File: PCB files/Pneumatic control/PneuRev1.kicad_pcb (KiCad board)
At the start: 2 copper layers, 154.1 x 77.3 mm, 76 parts, among them J1 SIG_IN, J2 BATT_IN, J3 PNEU, U1 OPA551, U10 OPA551, U11 OPA551, U12 OPA551, U13 OPA551, U2 OPA551, U3 OPA551, U4 OPA551, U5 OPA551, U6 OPA551, U7 OPA551, U8 OPA551, U9 OPA551

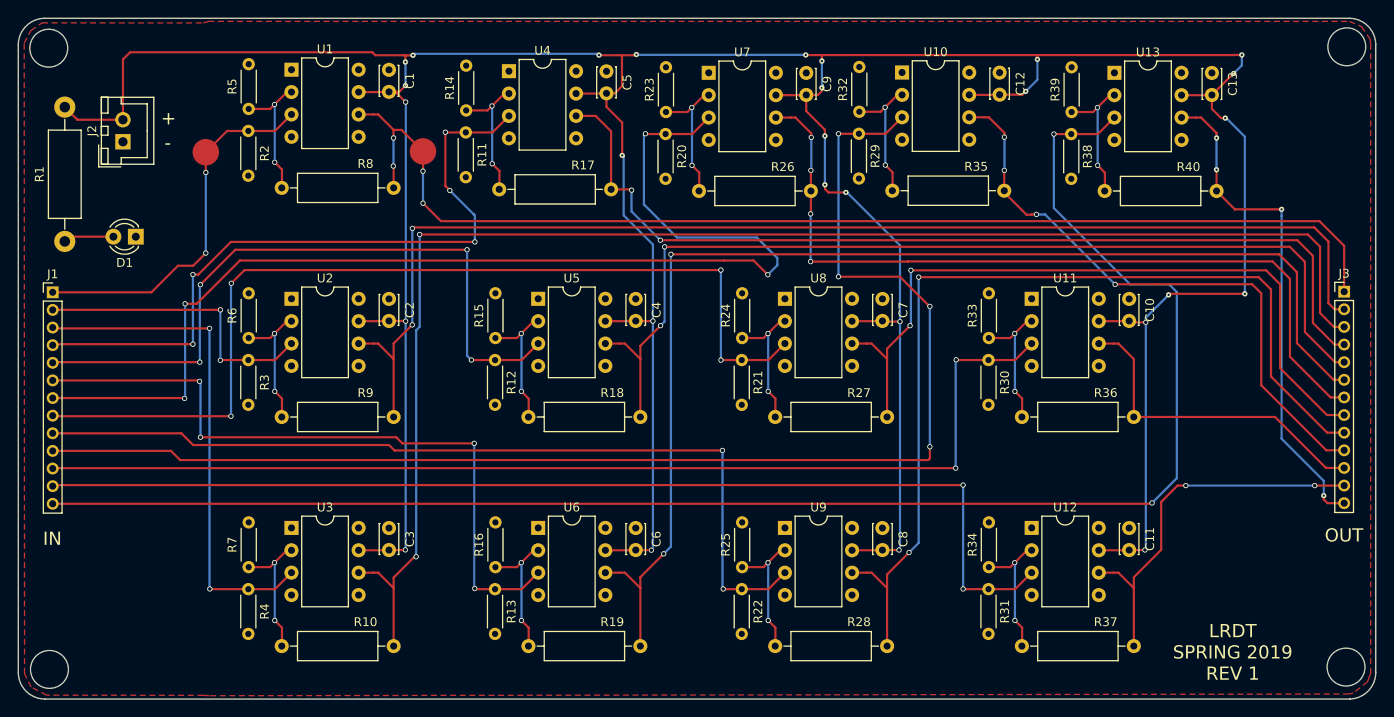
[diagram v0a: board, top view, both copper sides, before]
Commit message: 12/10/2019
-Selected battery molex connector footprint
-Read netlist
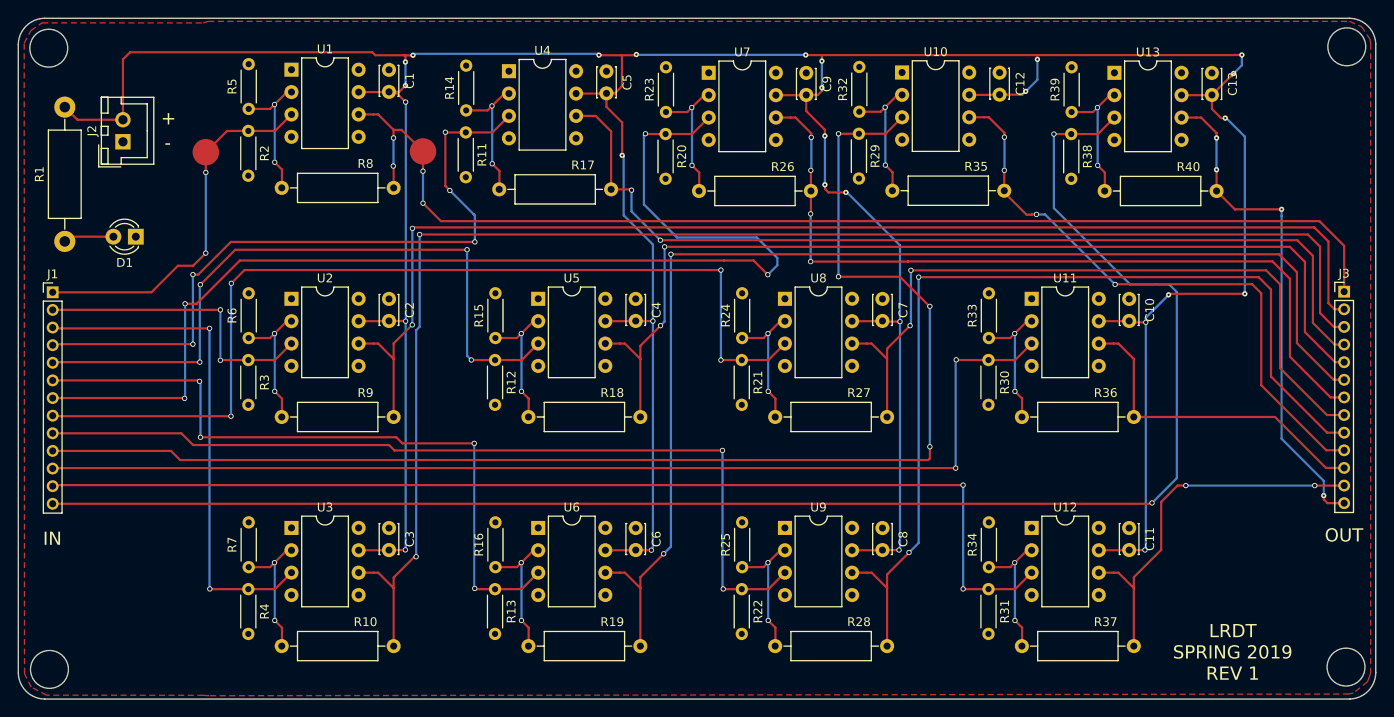
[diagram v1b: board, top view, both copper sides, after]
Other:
- outline, holes or cut-outs redrawn
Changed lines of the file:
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@@
-(kicad_pcb (version 4) (host pcbnew 4.0.7)
+(kicad_pcb (version 20171130) (host pcbnew "(5.1.2)-2")
   (general
-    (links 161)
-    (no_connects 53)
-    (area 65.792257 61.697777 219.999783 139.104441)
     (thickness 1.6)
     (drawings 13)
@@
     (zone_45_only no)
     (trace_min 0.2)
-    (segment_width 0.2)
-    (edge_width 0.15)
     (via_size 0.6)
     (via_drill 0.3)
@@
     (uvia_min_size 0.2)
     (uvia_min_drill 0.1)
+    (edge_width 0.15)
+    (segment_width 0.2)
     (pcb_text_width 0.3)
     (pcb_text_size 1.5 1.5)
@@
       (layerselection 0x00030_80000001)
       (usegerberextensions true)
+      (usegerberattributes false)
+      (usegerberadvancedattributes false)
+      (creategerberjobfile false)
       (excludeedgelayer true)
       (linewidth 0.100000)
@@
       (hpglpennumber 1)
       (hpglpenspeed 20)
-      (hpglpendiameter 15)
-      (hpglpenoverlay 2)
+      (hpglpendiameter 15.000000)
       (psnegative false)
       (psa4output false)
@@
       (drillshape 0)
       (scaleselection 1)
-      (outputdirectory ./))
+      (outputdirectory "./"))
   )
   (net 0 "")
@@
     (pad 1 np_thru_hole circle (at 0 0) (size 4.3 4.3) (drill 4.3) (layers *.Cu *.Mask))
   )
+  (gr_line (start 219.923261 64.673484) (end 219.924782 136.033093) (layer Edge.Cuts) (width 0.15))
   (gr_text OUT (at 216.31656 120.45442) (layer F.SilkS)
     (effects (font (size 1.5 1.5) (thickness 0.3)))
@@
     (effects (font (size 1.5 1.5) (thickness 0.3)))
   )
-  (gr_arc (start 216.903013 64.795378) (end 216.928413 61.772778) (angle 88.0744171) (layer Edge.Cuts) (width 0.15))
+  (gr_arc (start 216.903013 64.795378) (end 216.928413 61.772778) (angle 87.20739162) (layer Edge.Cuts) (width 0.15))
   (gr_arc (start 216.902182 136.007693) (end 219.924782 136.033093) (angle 87.91483468) (layer Edge.Cuts) (width 0.15))
-  (gr_arc (start 68.886487 136.011942) (end 68.86956 139.02944) (angle 88.23447828) (layer Edge.Cuts) (width 0.15))
+  (gr_arc (start 68.886487 136.011942) (end 68.87464 139.02944) (angle 88.33092298) (layer Edge.Cuts) (width 0.15))
   (gr_arc (start 68.889858 64.794547) (end 65.867258 64.769147) (angle 88.0744171) (layer Edge.Cuts) (width 0.15))
-  (gr_line (start 68.877138 139.02944) (end 216.98712 139.02944) (layer Edge.Cuts) (width 0.15))
-  (gr_line (start 219.92336 64.72428) (end 219.92476 136.03224) (layer Edge.Cuts) (width 0.15))
+  (gr_line (start 68.87718 139.02944) (end 216.98712 139.02944) (layer Edge.Cuts) (width 0.15))
   (gr_line (start 68.821293 61.7728) (end 216.92616 61.7728) (layer Edge.Cuts) (width 0.15))
   (gr_line (start 65.86982 136.08812) (end 65.86728 64.77254) (layer Edge.Cuts) (width 0.15))
